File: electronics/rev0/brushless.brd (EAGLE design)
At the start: 30 x 46 mm, 72 parts, among them Q1 BUK7Y12-40E, Q2 BUK7Y12-40E, Q3 BUK7Y12-40E, Q4 BUK7Y12-40E, Q5 BUK7Y12-40E, Q6 BUK7Y12-40E, X1 JST-XH-10-PIN-LONG-PAD

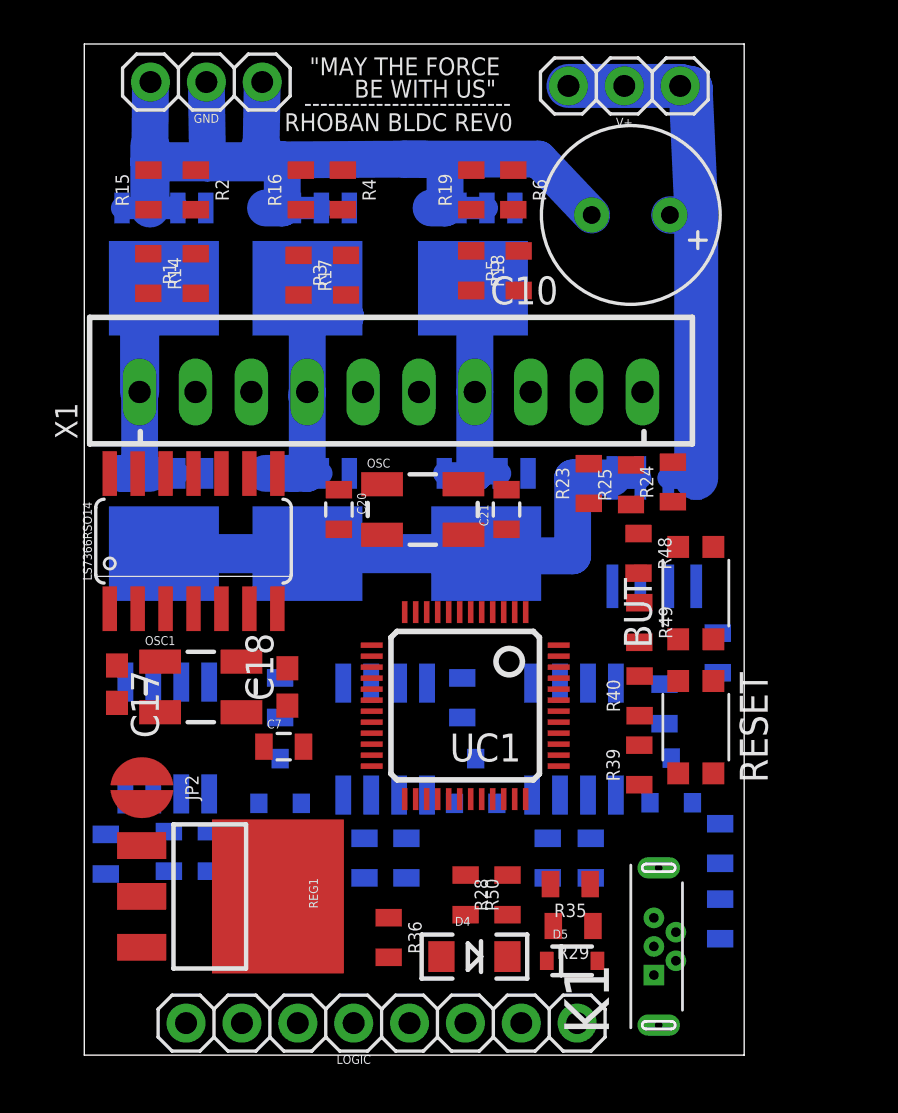
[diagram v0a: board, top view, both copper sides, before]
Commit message: rev0
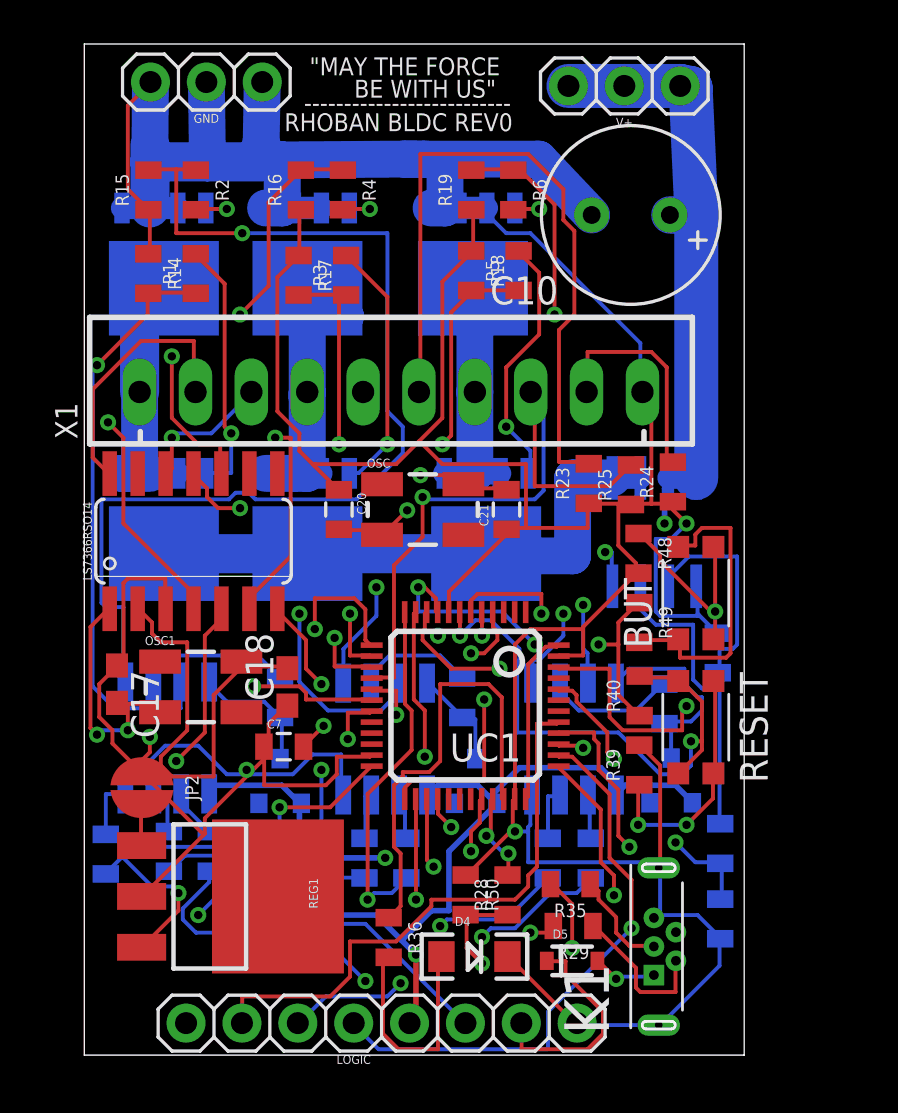
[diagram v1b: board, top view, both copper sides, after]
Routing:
- net GND: track 49.4 -> 268.7 mm, vias 0 -> 3
- net VCC: track 0.00 -> 86.1 mm, vias 0 -> 2
- net 3.3: track 0.00 -> 76.4 mm, vias 0 -> 6
- net U_HIGH: track 0.00 -> 58.5 mm, vias 0 -> 2
- net U_GATE_LOW: track 0.00 -> 49.1 mm, vias 0 -> 1
- net HALLU: track 0.00 -> 46.6 mm, vias 0 -> 1
- net U_LOW: track 0.00 -> 45.9 mm, vias 0 -> 2
- net VDRIVER: track 0.00 -> 44.1 mm, vias 0 -> 1
- net ENC_MISO: track 0.00 -> 41.8 mm, vias 0 -> 2
- net ENC_CS: track 0.00 -> 40.8 mm, vias 0 -> 3
- net INDEX: track 0.00 -> 36.6 mm, vias 0 -> 2
- net BUTTON: track 0.00 -> 35.8 mm, vias 0 -> 3
- net DISC: track 0.00 -> 32.7 mm, vias 0 -> 2
- net MISO: track 0.00 -> 32.7 mm, vias 0 -> 1
- net V_GATE_LOW: track 0.00 -> 32.6 mm, vias 0 -> 2
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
